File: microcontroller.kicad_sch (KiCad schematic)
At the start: 52 parts, among them J100 Conn_01x05_Pin, J101 Conn_01x03, J102 TC2030, J103 Screw_Terminal_01x02, J104 USB_C_Receptacle_USB2.0_16P, SW100 SW_Push, U100 STM32H563RITx, U101 AP2112K-3.3, U102 USBLC6-2SC6, Y100 16MHz

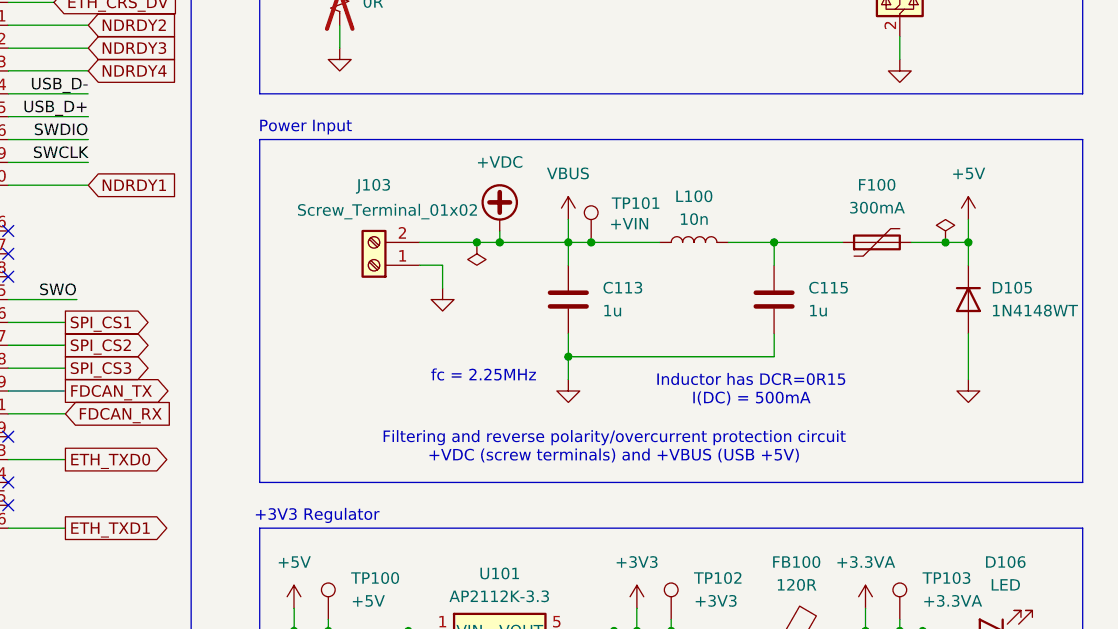
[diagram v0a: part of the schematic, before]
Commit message: Some changes to power circuitry, more layout
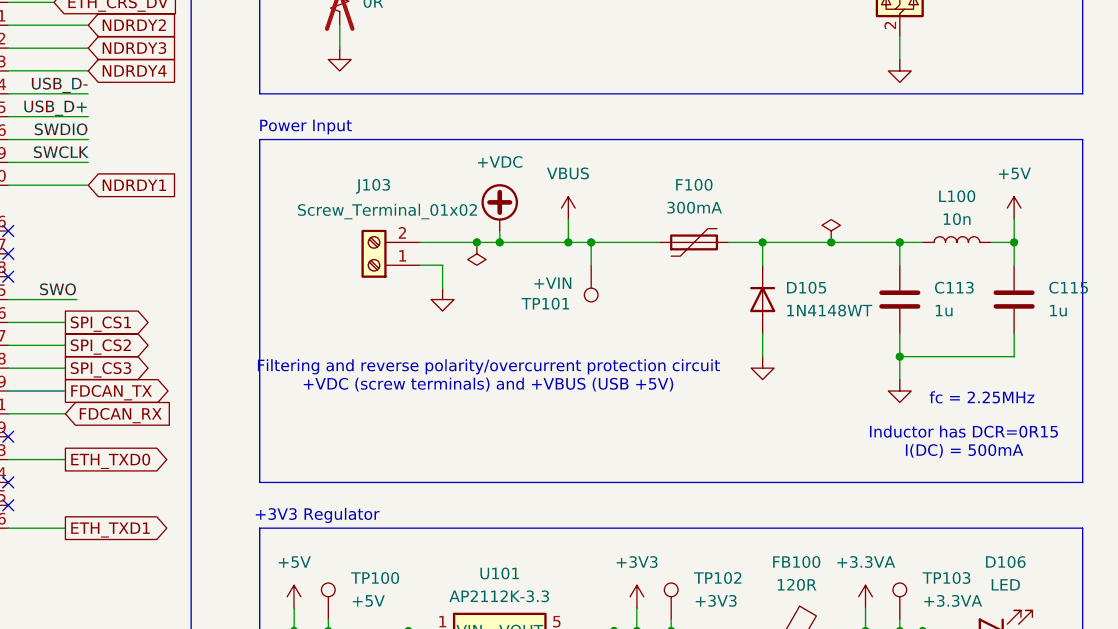
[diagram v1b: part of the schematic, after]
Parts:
- C100, C107, C109, C112, C113, C114, C115, C117: footprint Capacitor_SMD:C_0201_0603Metric -> Capacitor_SMD:C_0603_1608Metric
- C101, C102, C103, C104, C105, C106, C108, C110, C111, C116: footprint Capacitor_SMD:C_01005_0402Metric -> Capacitor_SMD:C_0402_1005Metric
- D106: footprint Capacitor_SMD:C_01005_0402Metric -> LED_SMD:LED_0402_1005Metric
- F100, FB100: footprint Capacitor_SMD:C_01005_0402Metric -> Capacitor_SMD:C_0603_1608Metric
- L100: footprint Inductor_SMD:L_0201_0603Metric -> Inductor_SMD:L_0603_1608Metric
- R100, R101, R102, R103, R104, R105, R106, R107, R108, R109: footprint Resistor_SMD:R_01005_0402Metric -> Resistor_SMD:R_0402_1005Metric
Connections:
- net +5V: now also C115.1, L100.2; no longer D105.1 (K), F100.2
- net +VDC: now also F100.1; no longer C113.1, L100.1
- new net: C113.1, D105.1 (K), F100.2, L100.1
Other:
- moved on the sheet: C113, C115, D105, F100, L100, TP101
